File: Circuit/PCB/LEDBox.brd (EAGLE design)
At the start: 28 x 28 mm, 12 parts, among them K1 D2F-5

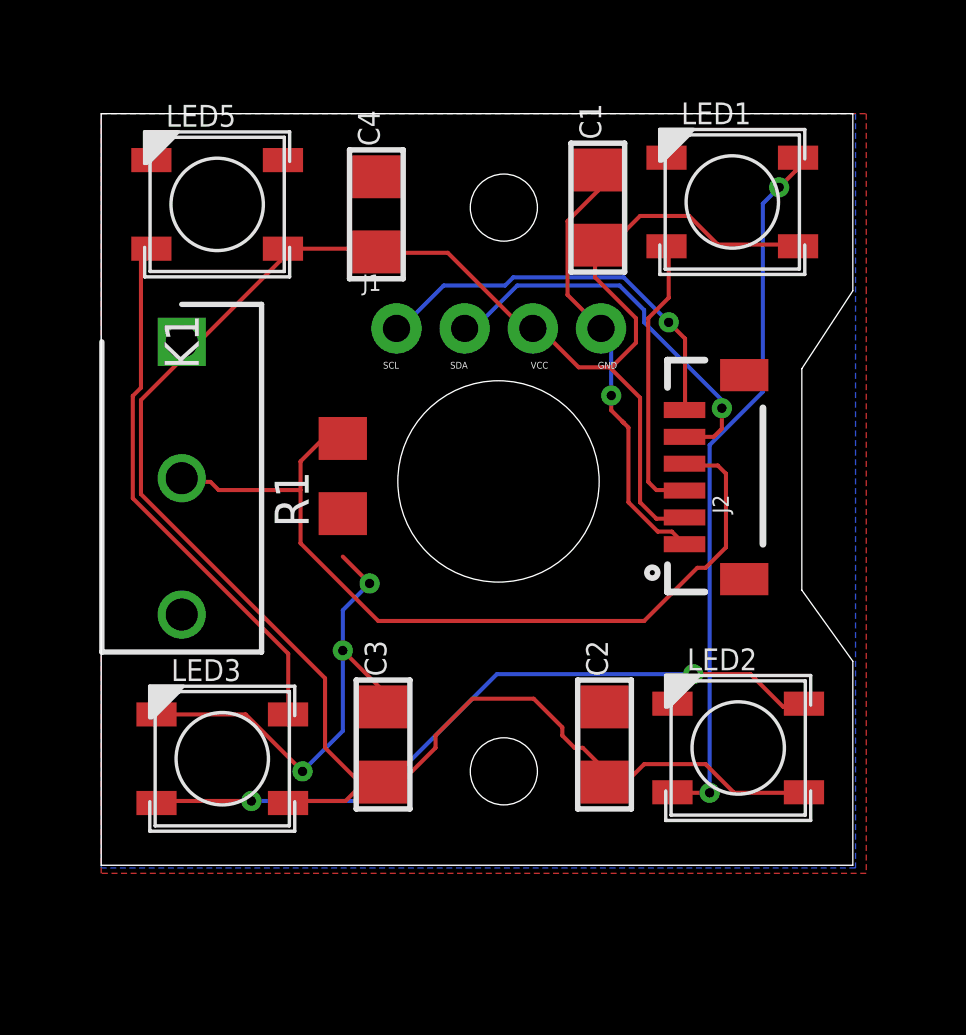
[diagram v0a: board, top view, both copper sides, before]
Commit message: PCB
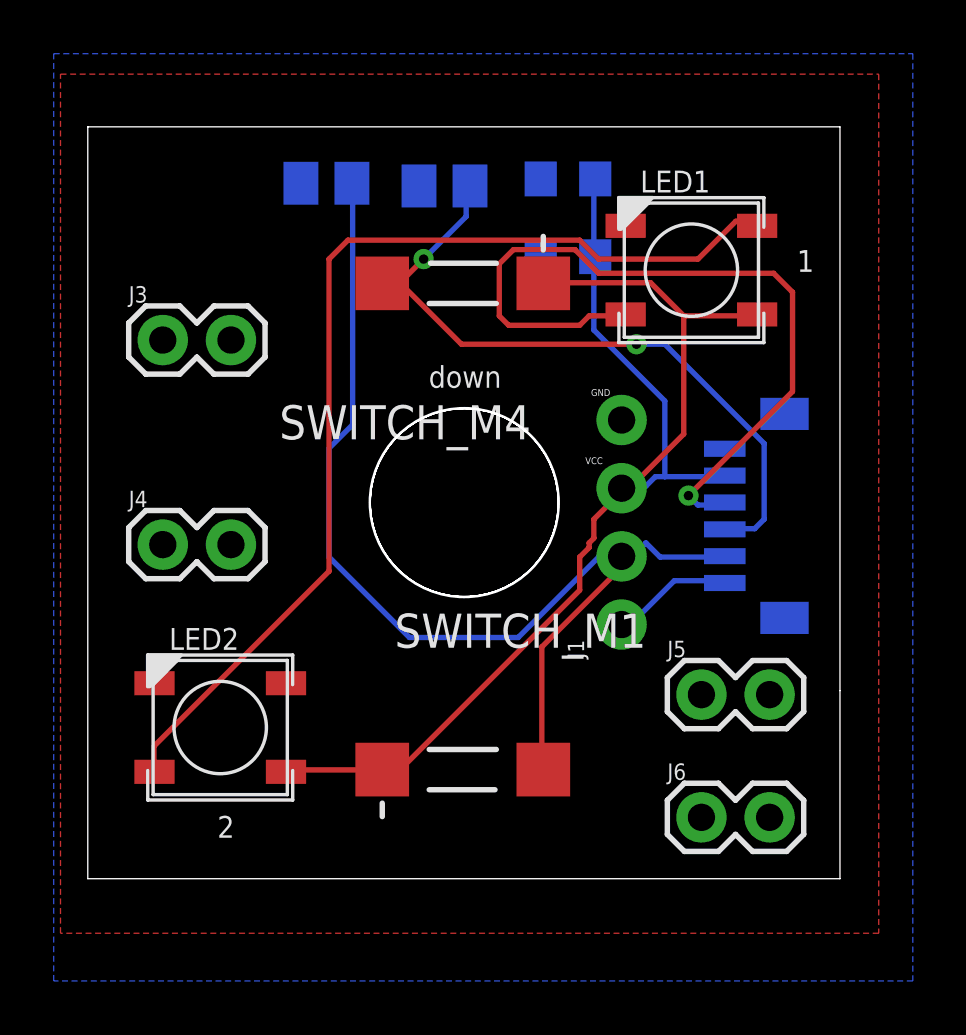
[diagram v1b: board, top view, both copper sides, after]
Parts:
- removed C3, C4: 0.1uf, microbuilder:1206
- removed K1: D2F-5, D2F-5:SHDR3W100P0X508_1X3_1280X580X5
- removed LED3, LED5: (no value), SK6812:LED5050
- added J3, J4, J5, J6: (no value), SparkFun-Connectors:1X02
- added R4: 10K, resistor:M0805
- added SWITCH_M1, SWITCH_M4: DTSM-3, switch-tact:DTSM-3
- C1, C2: device microbuilder:1206 -> rc-master-smd:C0805
- R1: value (none) -> 10K; device eagle-ltspice:R3216 -> resistor:M0805
- moved C2 21.1 mm to (17.9, 26.1), flipped to the bottom, turned to 180 degrees
- moved LED2 19.3 mm to (4.93, 5.63)
- moved J1 13.9 mm to (19.9, 9.47), turned to 90 degrees
- moved R1 10.9 mm to (8.89, 25.9), flipped to the bottom, turned to 180 degrees
- moved LED1 2.96 mm to (22.5, 22.7)
- moved C1 2.14 mm to (17.9, 23.2), flipped to the bottom, turned to 180 degrees
- moved J2 2.14 mm to (25.0, 13.5), flipped to the bottom, turned to 270 degrees
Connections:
- net LDIN renamed NEO_IN
- net SCL renamed DIO_IN
- removed net N$3: LED3.2-DOUT, LED5.4-DIN
- removed net N$6: K1.3
- removed net SDA: J1.2, J2.5
- removed net SDIN: J2.4, K1.2, R1.2
- new net SWD_IN: J2.4, R4.2, SWITCH_M4.2
- new net SWU_IN: J1.2, J2.5, R1.2, SWITCH_M1.2
- net GND: now also C1.1, C2.1, R4.1; no longer C1.2, C2.2, C3.2, C4.2, LED3.3-GND, LED5.3-GND
- net N$2: no longer LED3.4-DIN
- net VCC: now also C1.2, C2.2, SWITCH_M1.1, SWITCH_M4.1; no longer C1.1, C2.1, C3.1, C4.1, K1.1, LED3.1-VDD, LED5.1-VDD
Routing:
- net SWU_IN: track 0.00 -> 41.3 mm
- net VCC: track 86.7 -> 50.6 mm
- net GND: track 35.1 -> 0.00 mm, vias 4 -> 0
- net SDIN: track 32.2 -> 0.00 mm
- net N$2: track 26.7 -> 0.00 mm, vias 2 -> 0
- net SWD_IN: track 0.00 -> 26.6 mm, vias 0 -> 2
- net N$3: track 20.1 -> 0.00 mm
- net NEO_IN: track 10.6 -> 29.5 mm, vias 0 -> 1
- net SDA: track 14.9 -> 0.00 mm, vias 1 -> 0
- net N$1: track 26.4 -> 39.0 mm, vias 2 -> 0
- net DIO_IN: track 15.2 -> 4.56 mm, vias 1 -> 0
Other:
- outline, holes or cut-outs redrawn
- board text added: "1"
- board text added: "2"
- board text added: "down"
- board text removed: "SCL"
- board text removed: "SDA"
